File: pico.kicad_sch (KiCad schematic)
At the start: 35 parts, among them J101 Programming, J102 ???, J103 XT60, Q101 IRFS7434TRL7PP, U101 TPS7A2033PDBVR, U106 ADC124S051CIMM/NOPB

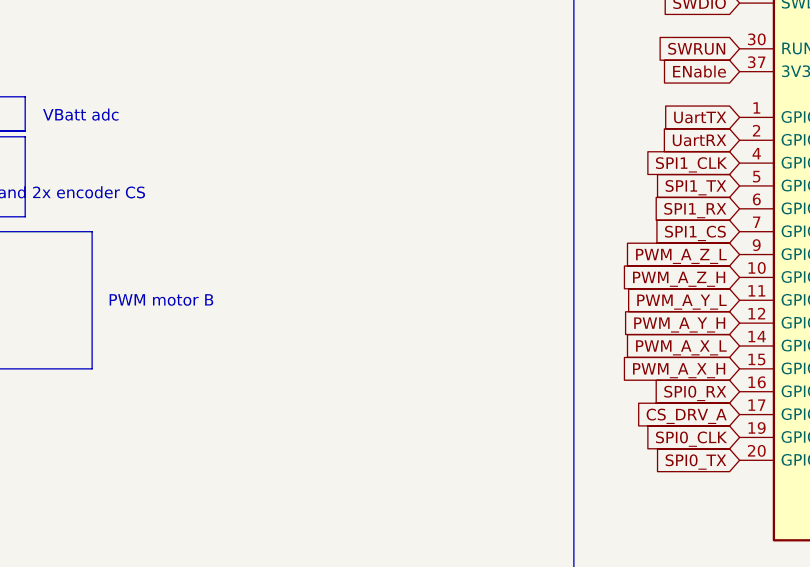
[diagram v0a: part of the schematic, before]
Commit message: ewdwad
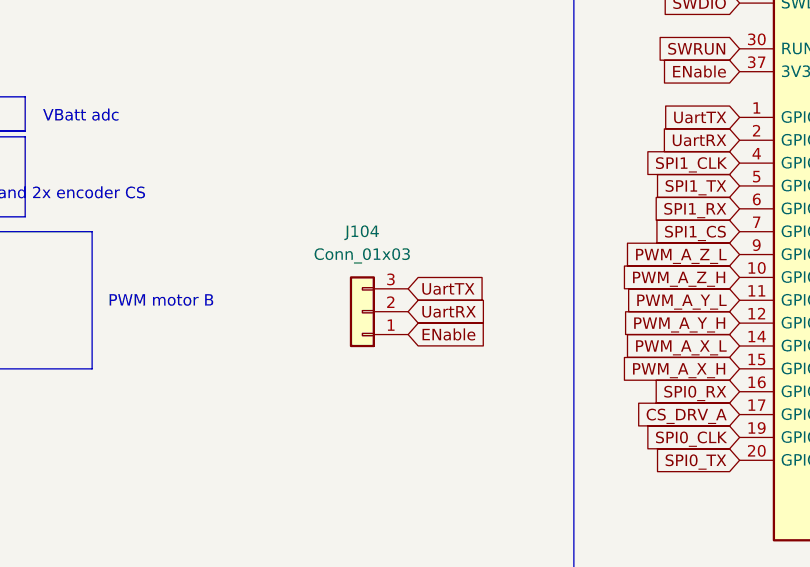
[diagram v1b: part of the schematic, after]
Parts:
- added J104: Conn_01x03, Connector_JST:JST_EH_B3B-EH-A_1x03_P2.50mm_Vertical, symbol Connector_Generic:Conn_01x03
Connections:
- net ENable: now also J104.1 (Pin_1)
- net UartRX: now also J104.2 (Pin_2)
- net UartTX: now also J104.3 (Pin_3)
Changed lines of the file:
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@@
 		)
 	)
+	(global_label "UartRX"
+		(shape input)
+		(at 31.75 66.04 0)
+		(fields_autoplaced yes)
+		(effects
+			(font
+				(size 1.27 1.27)
+			)
+			(justify left)
+		)
+		(property "Intersheetrefs" "${INTERSHEET_REFS}"
+			(at 41.2061 66.04 0)
+			(effects
+				(font
+					(size 1.27 1.27)
+				)
+				(justify left)
+				(hide yes)
+			)
+		)
+	)
 	(global_label "ADC1+"
 		(shape input)
@@
 		)
 	)
+	(global_label "ENable"
+		(shape input)
+		(at 31.75 68.58 0)
+		(fields_autoplaced yes)
+		(effects
+			(font
+				(size 1.27 1.27)
+			)
+			(justify left)
+		)
+		(property "Intersheetrefs" "${INTERSHEET_REFS}"
+			(at 41.2665 68.58 0)
+			(effects
+				(font
+					(size 1.27 1.27)
+				)
+				(justify left)
+				(hide yes)
+			)
+		)
+	)
+	(global_label "UartTX"
+		(shape input)
+		(at 31.75 63.5 0)
+		(fields_autoplaced yes)
+		(effects
+			(font
+				(size 1.27 1.27)
+			)
+			(justify left)
+		)
+		(property "Intersheetrefs" "${INTERSHEET_REFS}"
+			(at 40.9037 63.5 0)
+			(effects
+				(font
+					(size 1.27 1.27)
+				)
+				(justify left)
+				(hide yes)
+			)
+		)
+	)
 	(global_label "SPI1_CS"
 		(shape input)
@@
 					(unit 1)
 				)
+			)
+		)
+	)
+	(symbol
+		(lib_id "Connector_Generic:Conn_01x03")
+		(at 26.67 66.04 180)
+		(unit 1)
+		(exclude_from_sim no)
+		(in_bom yes)
+		(on_board yes)
+		(dnp no)
+		(fields_autoplaced yes)
+		(property "Reference" "J104"
+			(at 26.67 57.15 0)
+			(effects
+				(font
+					(size 1.27 1.27)
+				)
+			)
+		)
+		(property "Value" "Conn_01x03"
+			(at 26.67 59.69 0)
+			(effects
+				(font
+					(size 1.27 1.27)
+				)
+			)
+		)
+		(property "Footprint" "Connector_JST:JST_EH_B3B-EH-A_1x03_P2.50mm_Vertical"
+			(at 26.67 66.04 0)
+			(effects
+				(font
+					(size 1.27 1.27)
+				)
+				(hide yes)
+			)
+		)
+		(property "Datasheet" "~"
+			(at 26.67 66.04 0)
+			(effects
+				(font
+					(size 1.27 1.27)
+				)
+				(hide yes)
+			)
+		)
+		(property "Description" "Generic connector, single row, 01x03, script generated (kicad-library-utils/schlib/autogen/connector/)"
+			(at 26.67 66.04 0)
+			(effects
+				(font
+					(size 1.27 1.27)
+				)
+				(hide yes)
+			)
+		)
+		(pin "1"
+		)
+		(pin "3"
+		)
+		(pin "2"
+		)
+		(instances
+			(project ""
+				(path "/ee499c9f-2c44-4eb0-b36d-4920617b3177"
+					(reference "J104")
+					(unit 1)
+				)

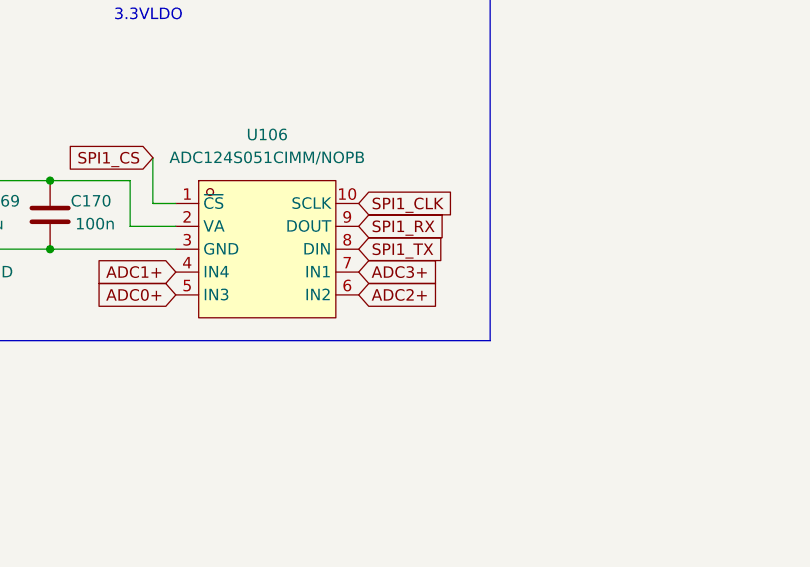
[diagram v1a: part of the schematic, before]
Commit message: wdawdawd
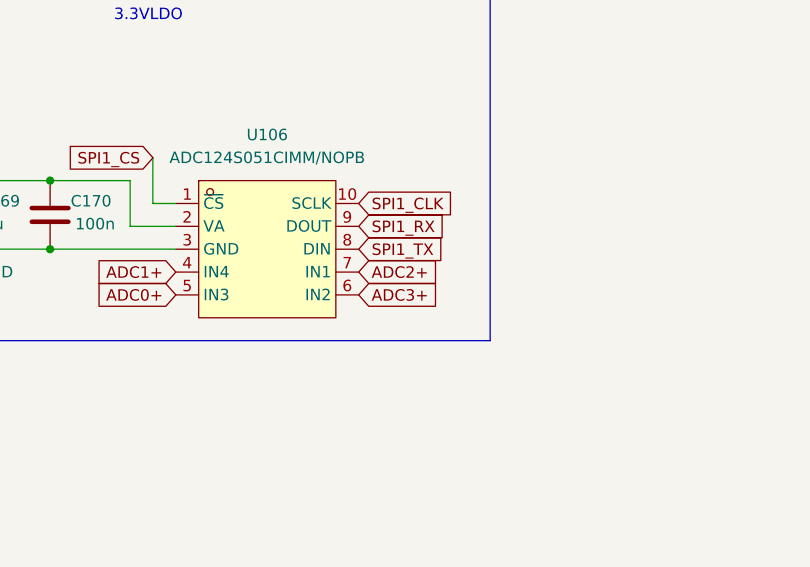
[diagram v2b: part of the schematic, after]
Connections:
- net ADC2+: now also U106.7 (IN1); no longer U106.6 (IN2)
- net ADC3+: now also U106.6 (IN2); no longer U106.7 (IN1)

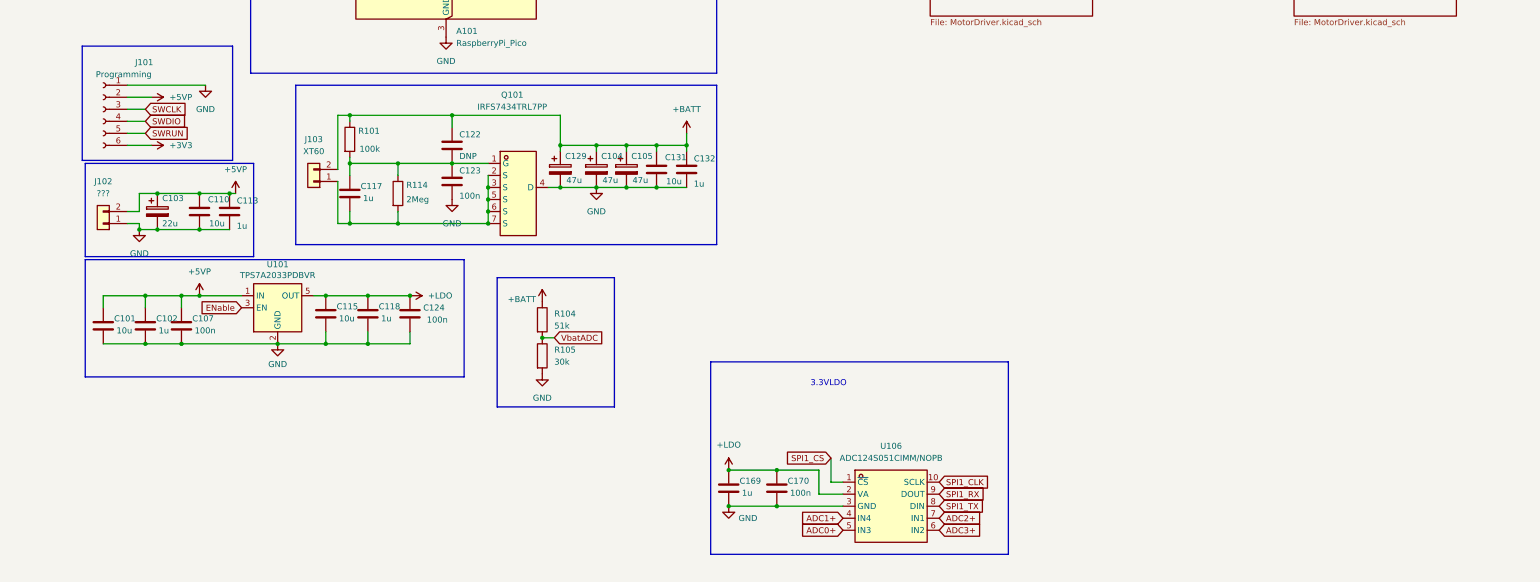
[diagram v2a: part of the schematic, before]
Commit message: why every commit needs a message
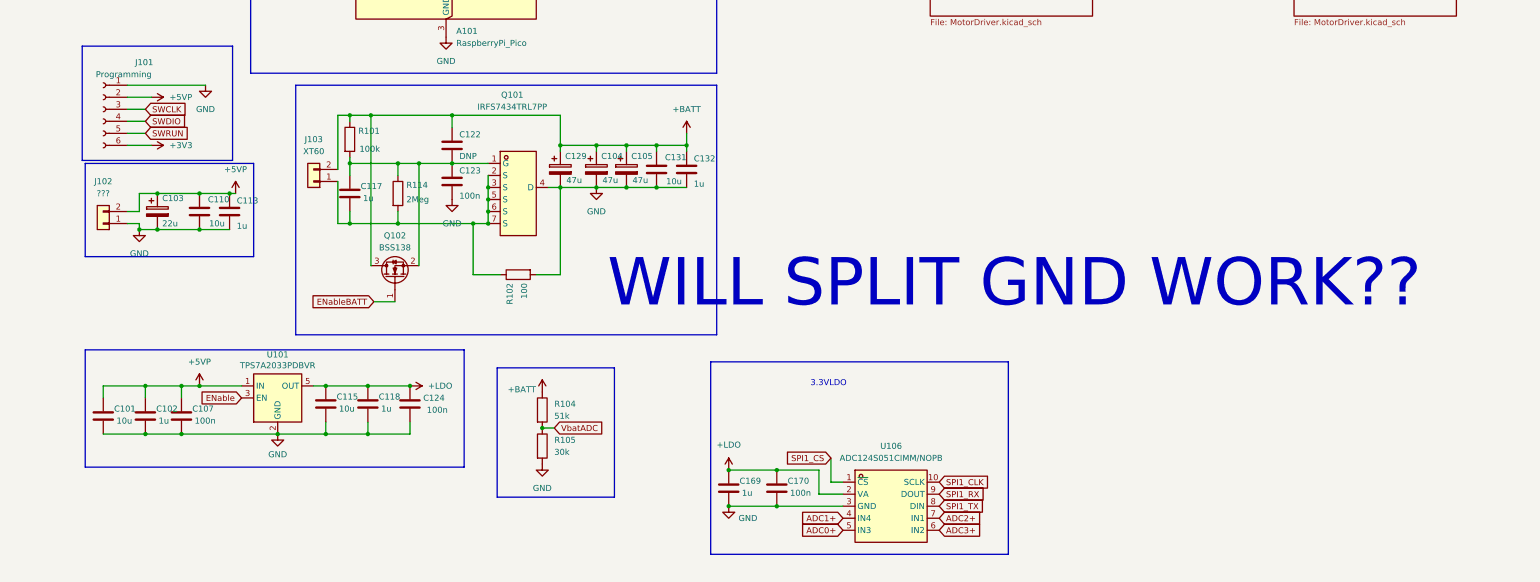
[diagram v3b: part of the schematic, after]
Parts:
- added Q102: BSS138, Package_TO_SOT_SMD:SOT-23, symbol Transistor_FET:BSS138
- added R102: 100, COMPONENTS:1206_Resistor, symbol Device:R
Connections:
- net +BATT: now also Q102.3 (D)
- net GND: now also R102.2
- net at C117.1, C122.2, C123.1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: now also Q102.2 (S)
- net at C117.2, J103.1 (Pin_1), Q101.2 (S)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: now also R102.1
- new net ENableBATT: Q102.1 (G)
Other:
- note added: "WILL SPLIT GND WORK??"
- moved on the sheet: C101, C102, C107, C115, C118, C124, R104, R105, U101

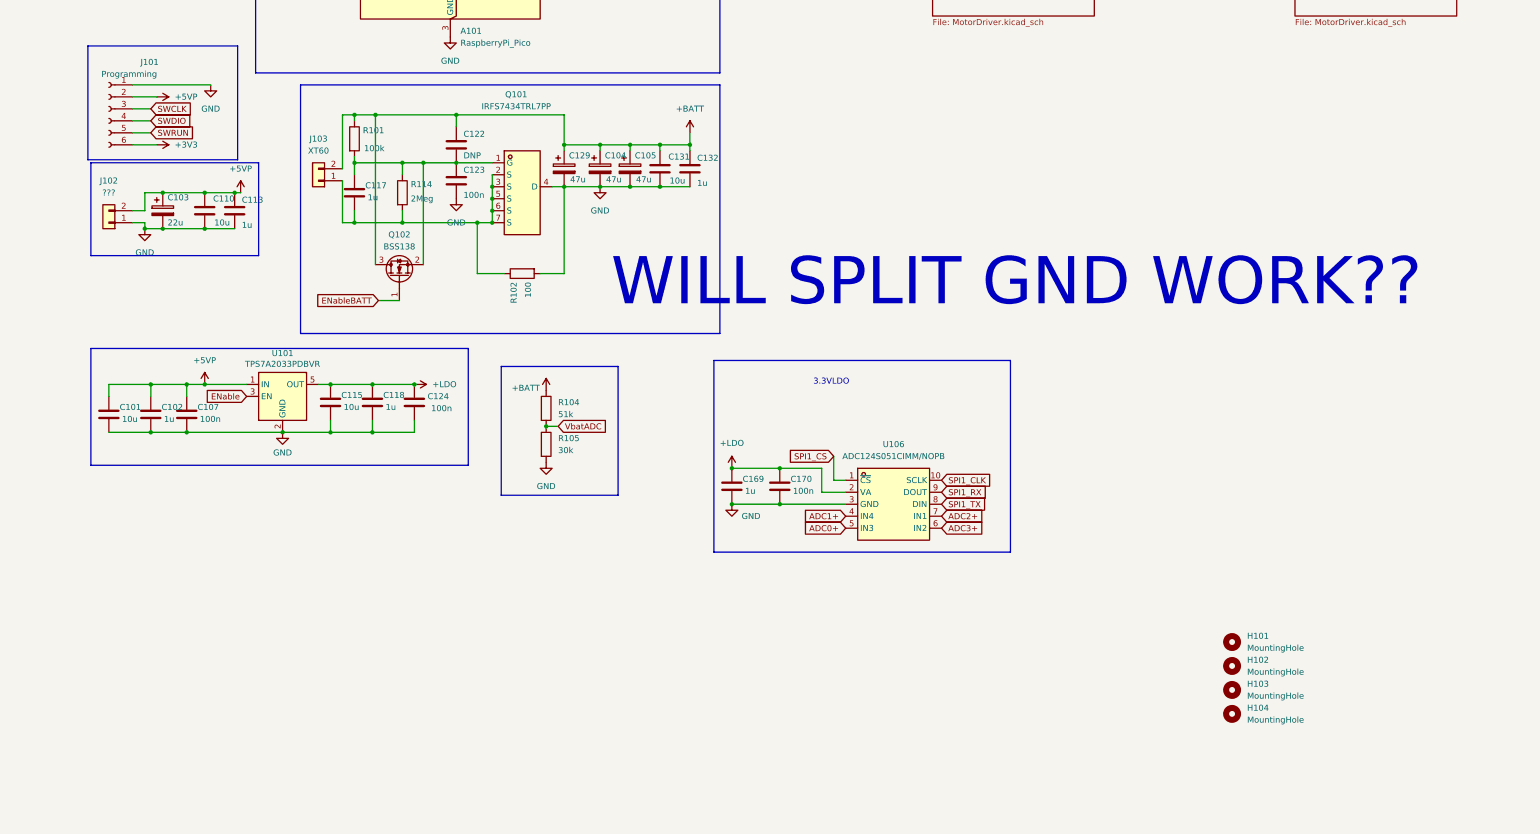
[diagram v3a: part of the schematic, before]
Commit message: Good progress
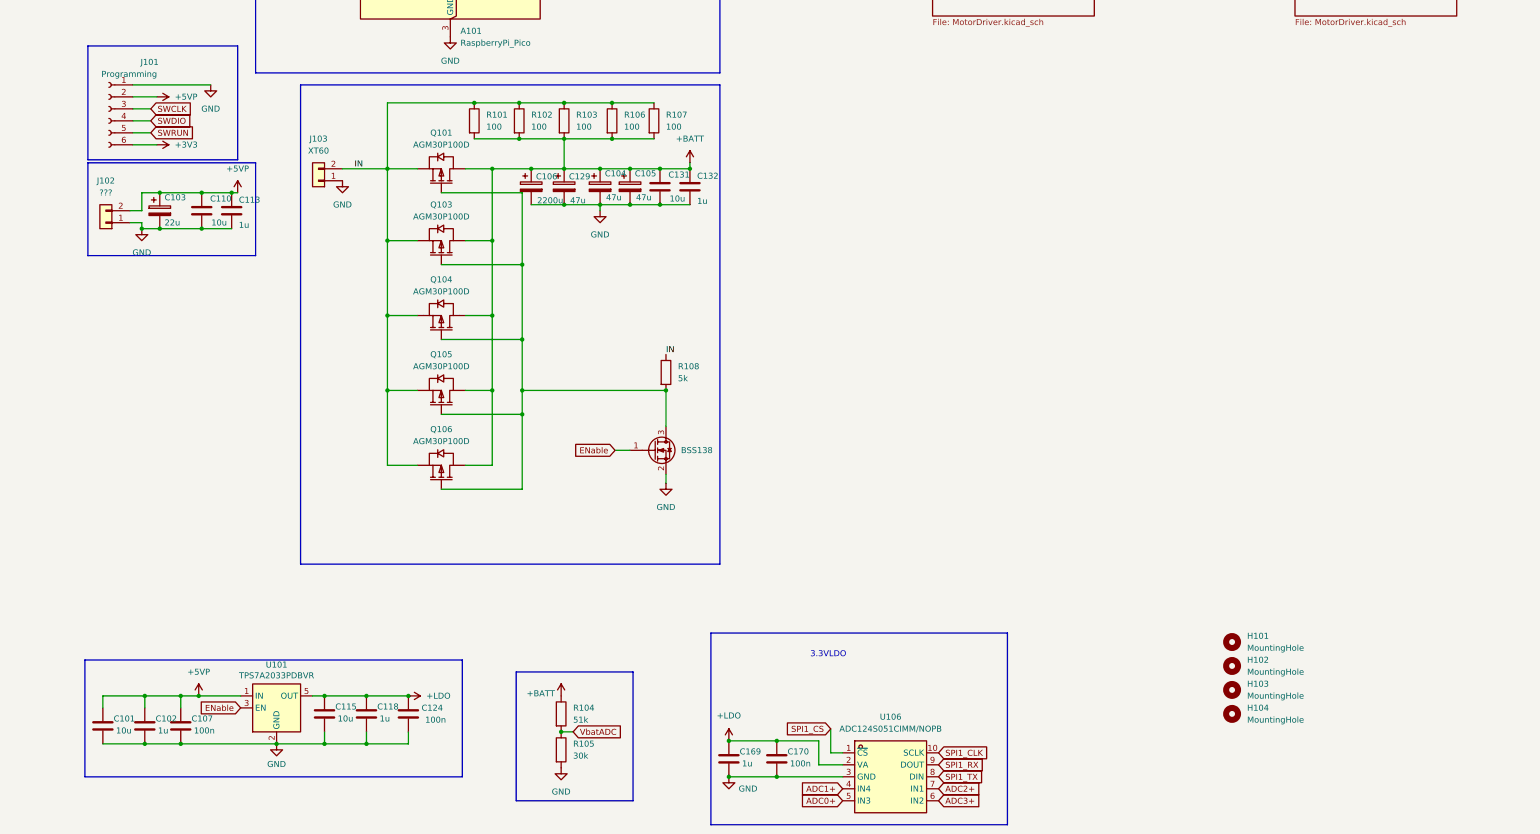
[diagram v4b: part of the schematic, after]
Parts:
- removed C117: 1u, COMPONENTS:1206_Resistor, symbol Device:C
- removed C122: DNP, COMPONENTS:1206_Resistor, symbol Device:C
- removed C123: 100n, COMPONENTS:1206_Resistor, symbol Device:C
- removed Q101: IRFS7434TRL7PP, JLCPCB_Transistors:D2PAK-7_L10.6-W9.6-P1.27-LS15.9-BR, symbol JLCPCB_Transistors:IRFS7434TRL7PP
- removed R114: 2Meg, COMPONENTS:1206_Resistor, symbol Device:R
- added C106: 2200u, Capacitor_THT:CP_Radial_D18.0mm_P7.50mm, symbol Device:C_Polarized
- added Q101, Q103, Q104, Q105, Q106: AGM30P100D, EasyEDA_Lib:TO-252-3_L6.6-W6.1-P4.57-LS9.9-BR-CW, symbol EasyEDA_Lib:AGM30P100D
- added R103, R106, R107: 100, COMPONENTS:1206_Resistor, symbol Device:R
- added R108: 5k, COMPONENTS:1206_Resistor, symbol Device:R
- R101: value 100k -> 100
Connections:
- net ENableBATT is gone; now on net ENable: Q102.1 (G)
- net +BATT: now also R101.2, R102.2, C106.1, Q101.2 (D), Q103.2 (D), Q104.2 (D), Q105.2 (D), Q106.2 (D), R103.2, R106.2, R107.2; no longer J103.2 (Pin_2), Q102.3 (D), R101.1
- net GND: now also J103.1 (Pin_1), Q102.2 (S), C106.2; no longer R102.2
- net IN: now reaches R102.1
- net IN: now also J103.2 (Pin_2), R101.1, Q101.3 (S), Q103.3 (S), Q104.3 (S), Q105.3 (S), Q106.3 (S), R103.1, R106.1, R107.1, R108.1; no longer J103.1 (Pin_1)
- new net: Q101.1 (G), Q102.3 (D), Q103.1 (G), Q104.1 (G), Q105.1 (G), Q106.1 (G), R108.2
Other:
- note removed: "WILL SPLIT GND WORK??"
- moved on the sheet: C101, C102, C103, C104, C105, C107, C110, C113, C115, C118, C124, C129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
